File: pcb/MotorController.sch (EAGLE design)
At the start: 7 parts

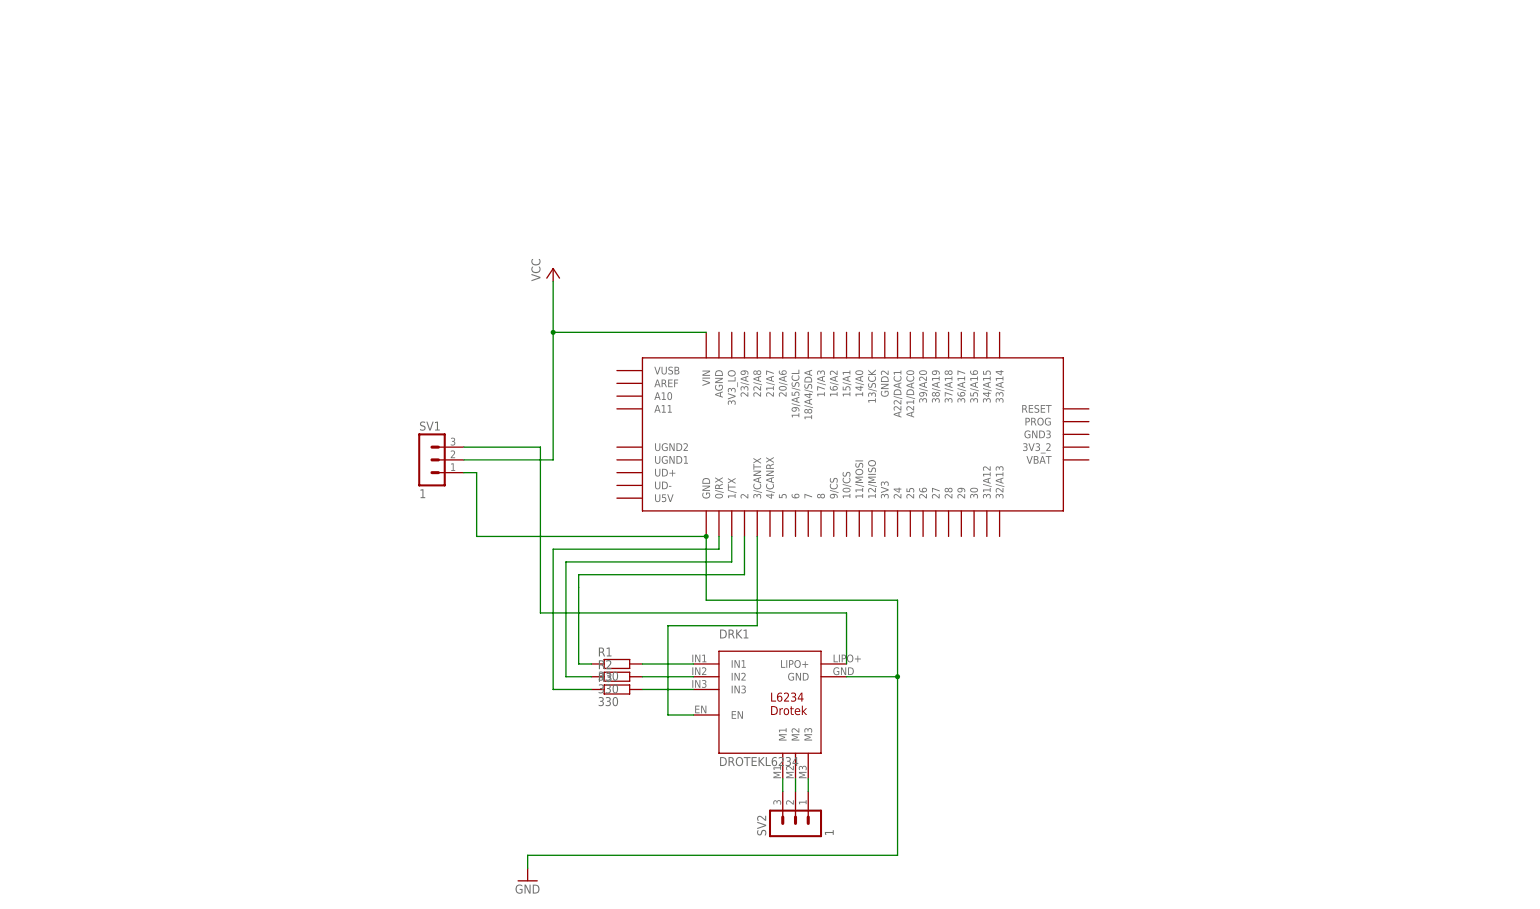
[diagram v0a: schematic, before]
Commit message: no message
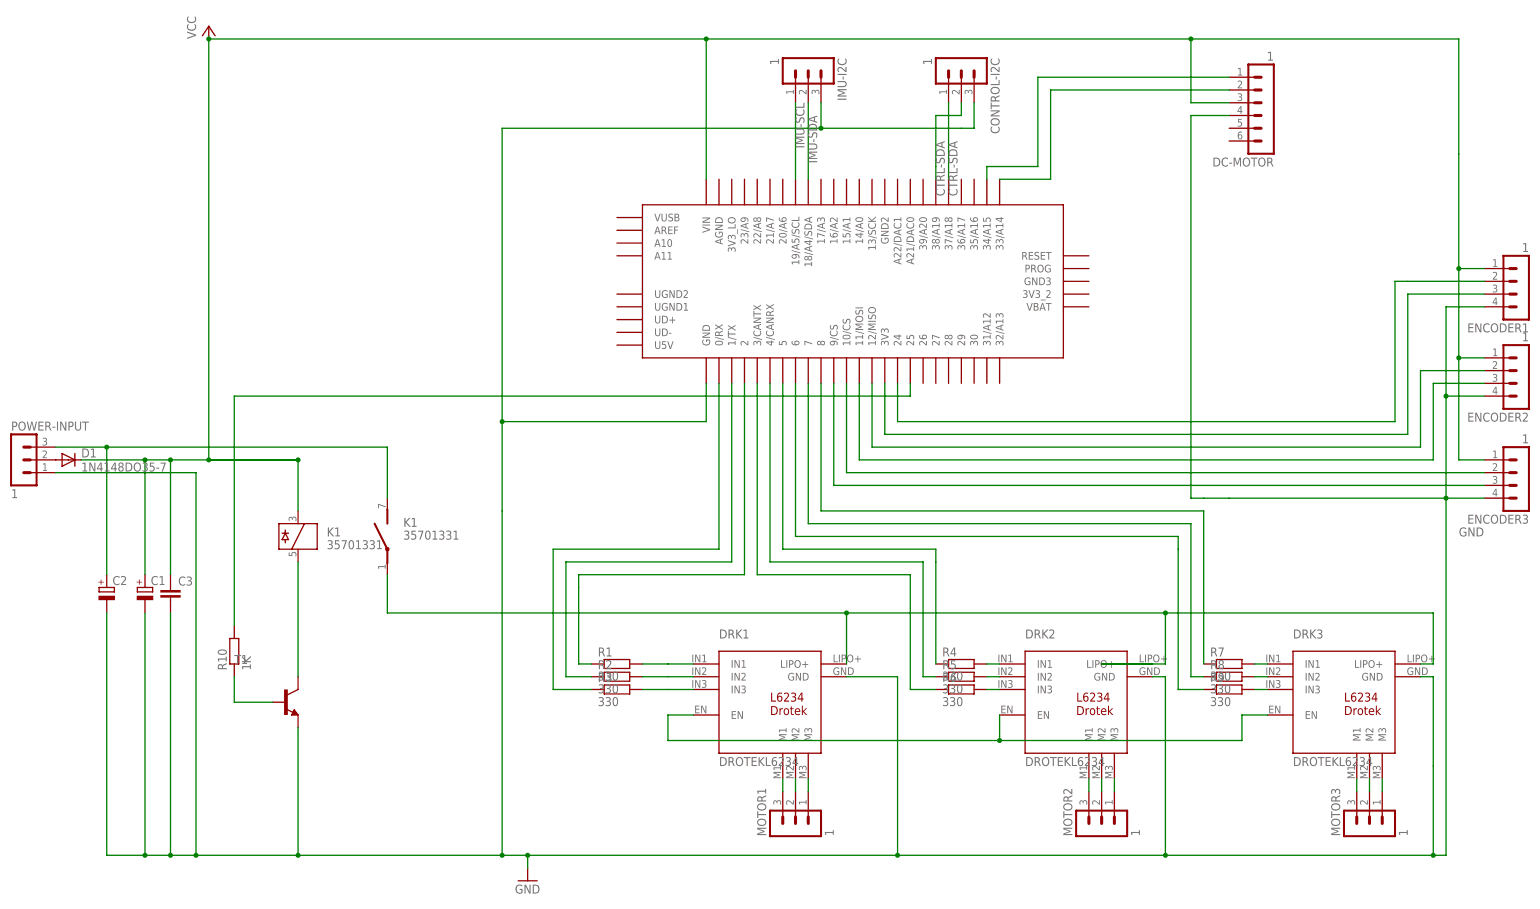
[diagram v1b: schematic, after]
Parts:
- removed SV1: 1, con-lstb:MA03-1
- added C1, C2: (no value), rcl:CPOL-EUE7.5-16
- added C3: (no value), capacitor-wima:C2.5/2
- added CONTROL-I2C, IMU-I2C, MOTOR2, MOTOR3, POWER-INPUT: 1, con-lstb:MA03-1
- added D1: 1N4148DO35-7, diode:1N4148DO35-7
- added DC-MOTOR: 1, con-lstb:MA06-1
- added DRK2, DRK3: DROTEKL6234, Drotek L6234:DROTEKL6234
- added ENCODER1, ENCODER2, ENCODER3: 1, con-lstb:MA04-1
- added K1: 35701331, relay:35701331
- added R10: 1K, resistor:R-EU_0204/7
- added R4, R5, R6, R7, R8, R9: 330, resistor:R-EU_0204/7
- added T1: (no value), transistor:-NPN-TO92
- renumbered SV2 to MOTOR1
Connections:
- new net CTRL-SDA: CONTROL-I2C.1, PRJ1.37/A18
- new net IMU-SCL: IMU-I2C.1, PRJ1.19/A5/SCL
- new net IMU-SDA: IMU-I2C.2, PRJ1.18/A4/SDA
- new net N$11: DRK2.IN1, R4.2
- new net N$13: DRK2.M1, MOTOR2.3
- new net N$14: DRK2.M2, MOTOR2.2
- new net N$15: DRK2.M3, MOTOR2.1
- new net N$16: DRK3.M1, MOTOR3.3
- new net N$17: DRK3.M2, MOTOR3.2
- new net N$18: DRK3.M3, MOTOR3.1
- new net N$19: DRK2.IN2, R5.2
- new net N$20: DRK2.IN3, R6.2
- new net N$21: PRJ1.3/CANTX, R6.1
- new net N$22: PRJ1.4/CANRX, R5.1
- new net N$23: PRJ1.5, R4.1
- new net N$24: DRK3.IN2, R8.2
- new net N$25: DRK3.IN1, R7.2
- new net N$26: DRK3.IN3, R9.2
- new net N$27: PRJ1.6, R9.1
- new net N$28: PRJ1.7, R8.1
- new net N$29: PRJ1.8, R7.1
- new net N$30: R10.1, T1.B
- new net N$31: K11.5, T1.C
- new net N$32: C2.+, K12.S, POWER-INPUT.3
- new net N$33: ENCODER3.3, PRJ1.9/CS
- new net N$34: ENCODER3.2, PRJ1.10/CS
- new net N$35: ENCODER2.3, PRJ1.11/MOSI
- new net N$36: ENCODER2.2, PRJ1.12/MISO
- new net N$37: ENCODER1.3, PRJ1.3V3
- new net N$38: ENCODER1.2, PRJ1.24
- new net N$39: D1.A, POWER-INPUT.2
- new net N$40: DC-MOTOR.2, PRJ1.33/A14
- new net N$41: DC-MOTOR.1, PRJ1.34/A15
- new net N$42: PRJ1.25, R10.2
- new net N$43: CONTROL-I2C.2, PRJ1.38/A19
- net GND: now also C1.-, C2.-, C3.2, CONTROL-I2C.3, DC-MOTOR.4, DRK2.GND, DRK3.GND, ENCODER1.4, ENCODER2.4, ENCODER3.4, IMU-I2C.3, POWER-INPUT.1, T1.E; no longer SV1.1
- net N$10: now also DRK2.EN, DRK3.EN; no longer PRJ1.3/CANTX
- net N$12: now also DRK2.LIPO+, DRK3.LIPO+, K12.P; no longer SV1.3
- net VCC: now also C1.+, C3.1, D1.C, DC-MOTOR.3, ENCODER1.1, ENCODER2.1, ENCODER3.1, K11.3; no longer SV1.2
